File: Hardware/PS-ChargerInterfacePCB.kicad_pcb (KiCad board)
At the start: 2 copper layers, 74.2 x 79.4 mm, 136 parts, among them IC1 TPS613771RYHR, IC2 LM74502HDDFR, IC3 LM74502HDDFR, J1 ElconConn, J2 SFH11-PBPC-D05-ST-BK, J3 BPSConn, J5 Estop 3, J6 BuzzConn, J7 105314-1110, J8 EVSE Conn, J9 ElconConn, Q1 NVMFWS1D7N04XMT1G, Q10 NVMFWS1D7N04XMT1G, Q11 NVMFWS1D7N04XMT1G, Q13 IRLML0030TRPBF, Q2 NVMFWS1D7N04XMT1G, Q4 IRLML0030TRPBF, Q5 IRLML0030TRPBF, Q6 IRLML0030TRPBF, Q7 IRLML0030TRPBF, Q8 IRLML0030TRPBF, U1 LeaderSOM, U2 4A

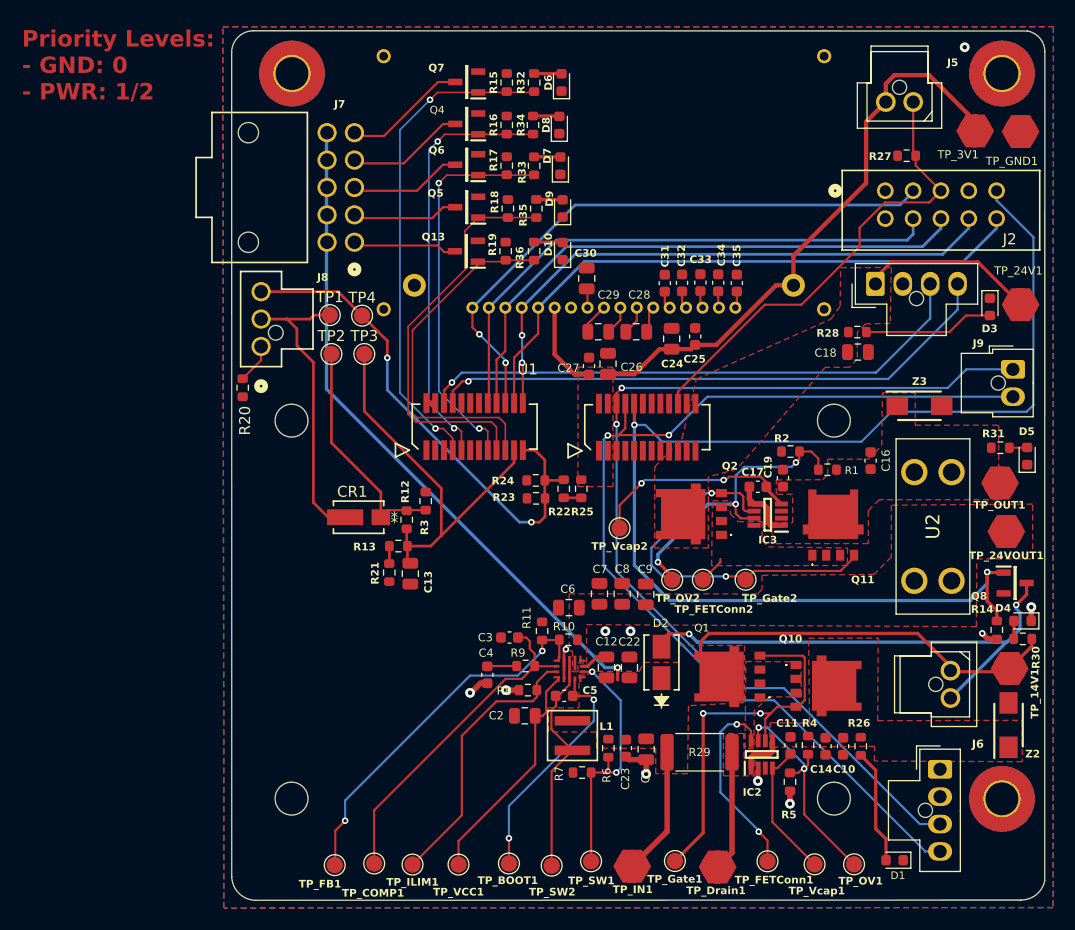
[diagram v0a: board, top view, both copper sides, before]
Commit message: Layout again
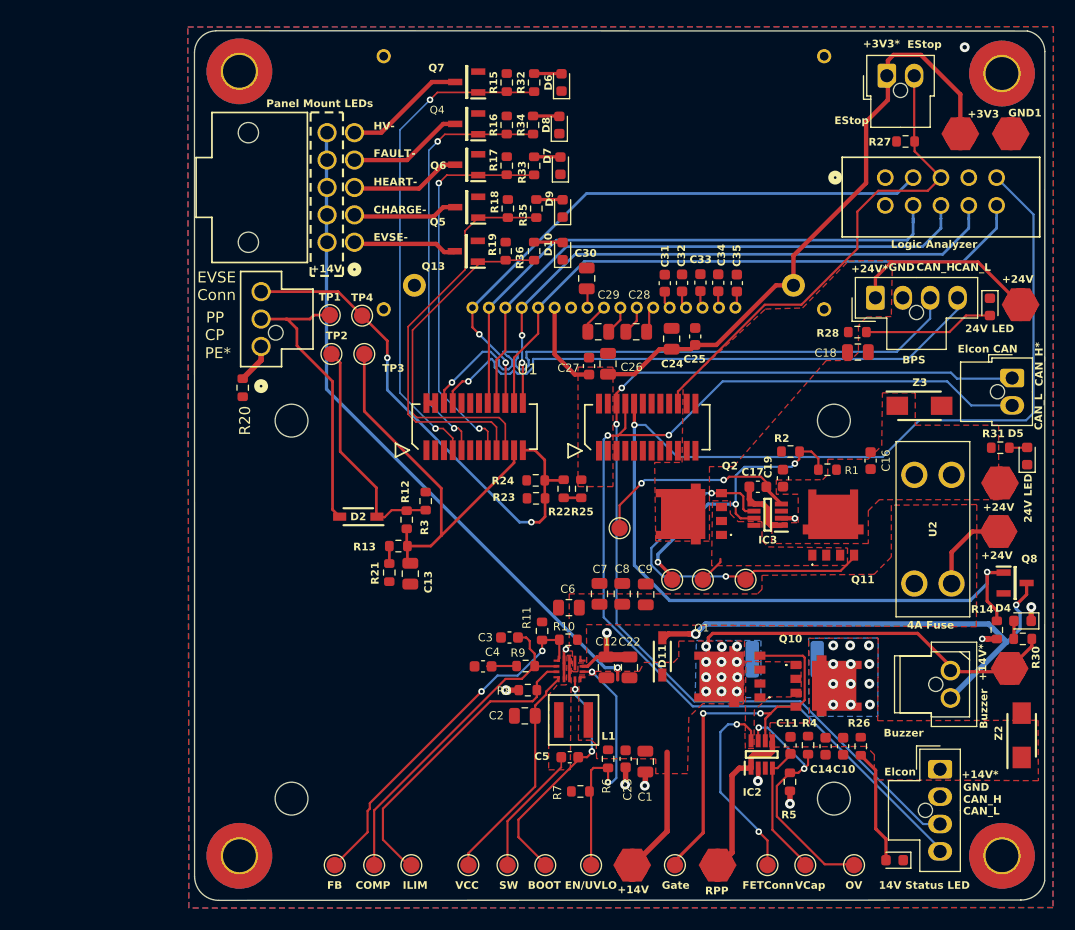
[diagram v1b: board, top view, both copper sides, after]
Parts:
- removed CR1: V8PAM10S-M3/I, V8PAM10S-M3-I:CR_10S-M3&slash_I_VIS
- removed J5: Estop 3, 153091202:1053091202
- added D11: 1N5819HW-7-F, 1N5819HW-7-F:SOD3716X145N, F.Cu at (101.4, 98.6)
- added Estop1: EStop Conn, UTSVT_Connectors:Molex_Nano-Fit_105309-xx02_1x02_P2.50mm_Vertical, F.Cu at (121.9, 45.6)
- added H3: MountingHole, MountingHole:MountingHole_3mm_Pad_TopBottom, F.Cu at (62.8, 116.8)
- 24V LED: renamed from D3
- D2: value D_Schottky -> 1N5819HW-7-F; footprint SK32A_LTP:SDO_DO-214AC-SMA_MCE -> 1N5819HW-7-F:SOD3716X145N
- R29: moved to B.Cu
- moved D2 30.7 mm to (73.7, 85.8), turned to 180 degrees
- moved R29 11.5 mm to (112.6, 98.9)
- moved C5 5.62 mm to (93.0, 107.8)
- moved H3 5.20 mm to (132.4, 116.8)
- moved H1 4.80 mm to (62.8, 45.2)
- moved SW1 4.03 mm to (87.3, 117.7)
- moved BOOT1 3.32 mm to (90.7, 117.7)
- moved R7 1.73 mm to (93.9, 110.9)
- moved Z2 1.52 mm to (134.2, 105.8)
- moved L1 1.43 mm to (93.3, 104.4), turned to 180 degrees
- moved +3V3 1.38 mm to (128.6, 50.9)
- moved R27 1.30 mm to (123.6, 51.6)
- moved Elcon2 1.27 mm to (123.9, 66.1)
- moved Logic_Analyzer1 1.20 mm to (121.8, 54.9)
- moved C1 1.13 mm to (99.8, 108.2)
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- renumbered TP_14V1 to +14V1, TP_IN1 to +14V2, TP_24V1 to +24V1, TP_24VOUT1 to +24V_IN1, TP_3V1 to +3V3, TP_OUT1 to 24V_OUT1, TP_BOOT1 to BOOT1, J6 to Buzzer1, TP_COMP1 to COMP1, TP_SW1 to EN/UVLO1, J8 to EVSE1, J1 to Elcon1, J3 to Elcon2, TP_FB1 to FB1, TP_GND1 to GND1, TP_Gate1 to Gate1, TP_Gate2 to Gate2, TP_ILIM1 to ILIM1, J2 to Logic_Analyzer1, TP_OV1 to OV1, TP_OV2 to OV2, J7 to Panel_LED801, TP_Drain1 to RPP_EN1, TP_SW2 to SW1, TP_VCC1 to VCC1, TP_Vcap1 to Vcap1, TP_Vcap2 to Vcap2
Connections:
- net /14V-24V Boost Converter/PostL1 renamed /14V-24V Boost Converter/SW
- D2 pad 1: +14V -> Net-(D2-K)
- D2 pad 2: /Buzzer/Buzz_Drain -> /EVSE_CP
- R12 pad 1: Net-(CR1-Pad1) -> Net-(D2-K)
- R3 pad 1: Net-(CR1-Pad1) -> Net-(D2-K)
- TP2 pad 1: Net-(CR1-Pad1) -> Net-(D2-K)
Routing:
- net Net-(D2-K): track 0.00 -> 21.3 mm
- net Net-(CR1-Pad1): track 21.1 -> 0.00 mm
- net /14V-24V Boost Converter/SW: track 20.4 -> 11.8 mm
- net /14V-24V Boost Converter/24V_Out_Fuse: track 0.00 -> 8.39 mm
- net /CarCAN_H: track 51.0 -> 58.0 mm
- net +3.3V: track 59.8 -> 64.5 mm
- net /ElconCAN_L: track 95.2 -> 99.5 mm
- net GND: track 17.7 -> 20.7 mm
- net /14V-24V Boost Converter/ILIM: track 25.5 -> 28.3 mm
- net /BuzzPWM: track 115.7 -> 118.5 mm
- net /Power14V/OV: track 20.7 -> 23.4 mm
- net /Estop: track 42.8 -> 45.5 mm
- net /CarCAN_L: track 52.2 -> 54.4 mm
- net /ElconCAN_H: track 92.4 -> 94.5 mm
- net /Display_RES: track 51.7 -> 53.2 mm
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- added copper zone on B.Cu, net +14V
- added copper zone on F.Cu, net /14V-24V Boost Converter/SW
- added copper zone on B.Cu, net /14V_IN
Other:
- board size 74.2 x 79.4 mm -> 77.6 x 79.4 mm
- board text added: "+14V"
- board text added: "+14V*"
- board text added: "+24V"
- board text added: "+24V*"
- board text added: "+3V3*"
- board text added: "14V Status LED"
- board text added: "24V LED"
- board text added: "4A Fuse"
- board text added: "BOOT"
- board text added: "BPS"
- board text added: "Buzzer"
- board text added: "CAN_H"
- board text added: "CAN_H*"
- board text added: "CAN_L"
- board text added: "CHARGE-"
- board text added: "COMP"
- board text added: "CP"
- board text added: "EN/UVLO"
- board text added: "EStop"
- board text added: "EVSE Conn"
- board text added: "EVSE-"
- board text added: "Elcon"
- board text added: "Elcon CAN"
- board text added: "FAULT-"
- board text added: "FB"
- board text added: "FETConn"
- board text added: "GND"
- board text added: "Gate"
- board text added: "HEART-"
- board text added: "HV-"
- board text added: "ILIM"
- board text added: "Logic Analyzer"
- board text added: "OV"
- board text added: "PE*"
- board text added: "PP"
- board text added: "Panel Mount LEDs"
- board text added: "RPP"
- board text added: "SW"
- board text added: "VCC"
- board text added: "VCap"
- board text removed: "Priority Levels: - GND: 0 - PWR: 1/2"
